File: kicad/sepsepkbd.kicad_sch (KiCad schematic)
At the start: 47 parts, among them J1 MJ-4PP-9, J2 Conn_01x04_Socket, J3 Conn_01x04_Socket, SW1 SW_PUSH, SW10 SW_PUSH, SW11 SW_PUSH, SW12 SW_PUSH, SW13 SW_PUSH, SW14 SW_PUSH, SW15 SW_PUSH, SW16 SW_PUSH, SW17 SW_PUSH, SW18 SW_PUSH, SW19 SW_PUSH, SW2 SW_PUSH, SW20 SW_PUSH, SW21 SW_PUSH, SW3 SW_PUSH, SW4 SW_PUSH, SW5 SW_PUSH, SW6 SW_PUSH, SW7 SW_PUSH, SW8 SW_PUSH, SW9 SW_PUSH, U1 ProMicro

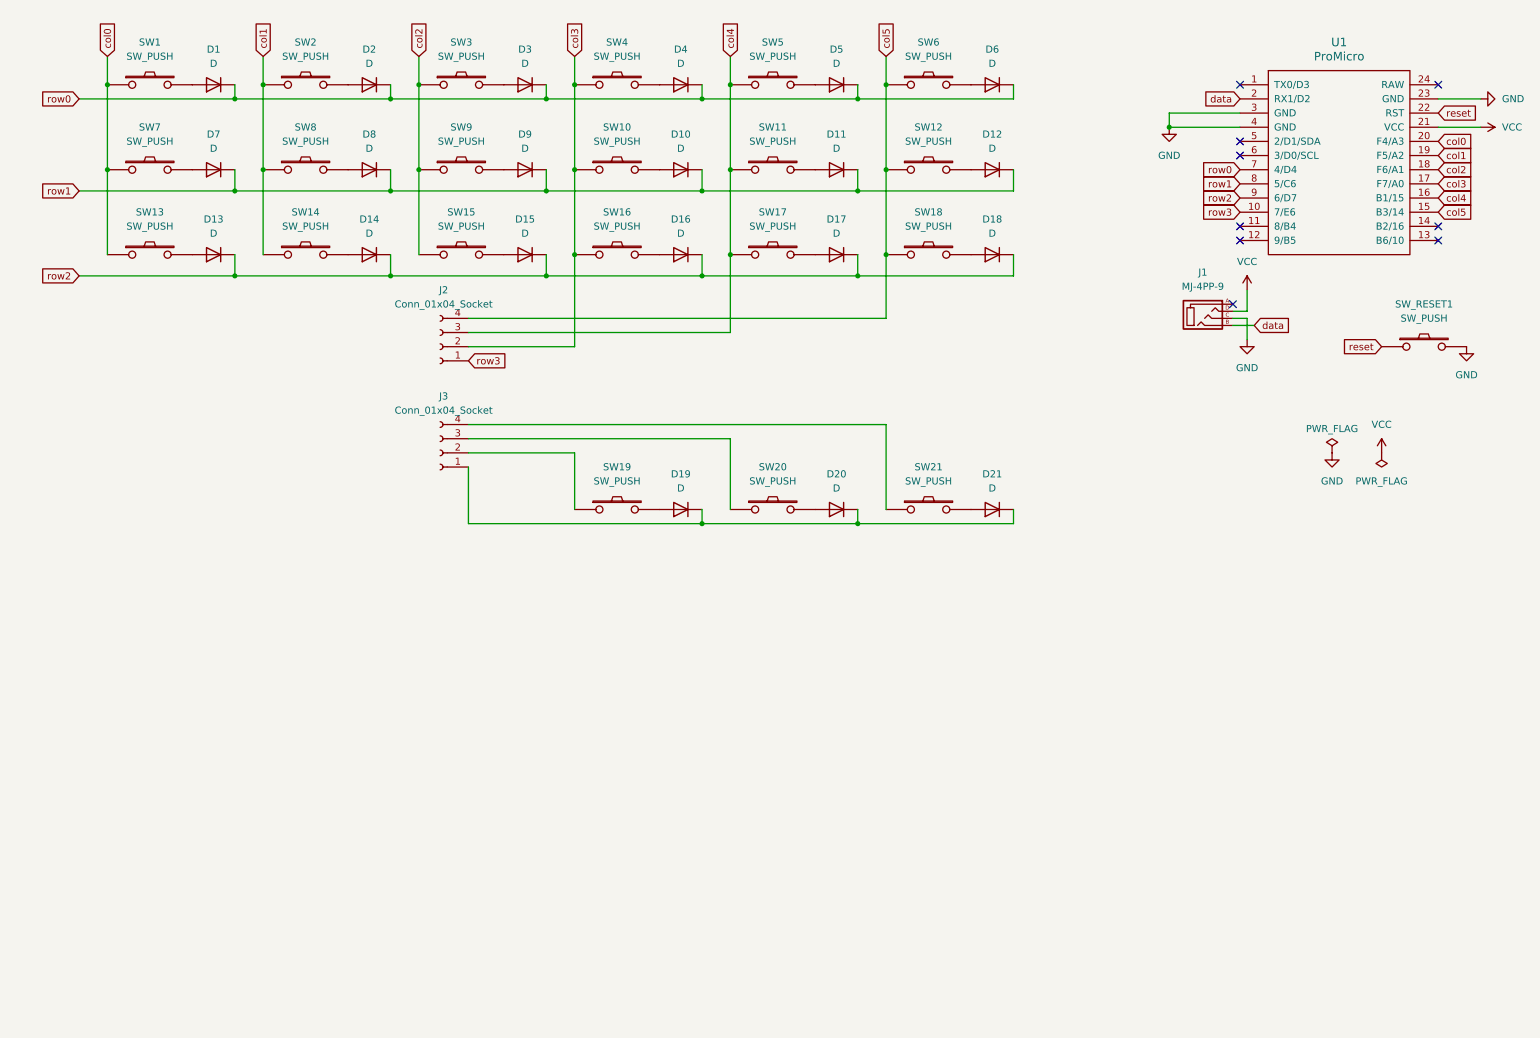
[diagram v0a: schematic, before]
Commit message: 2.1
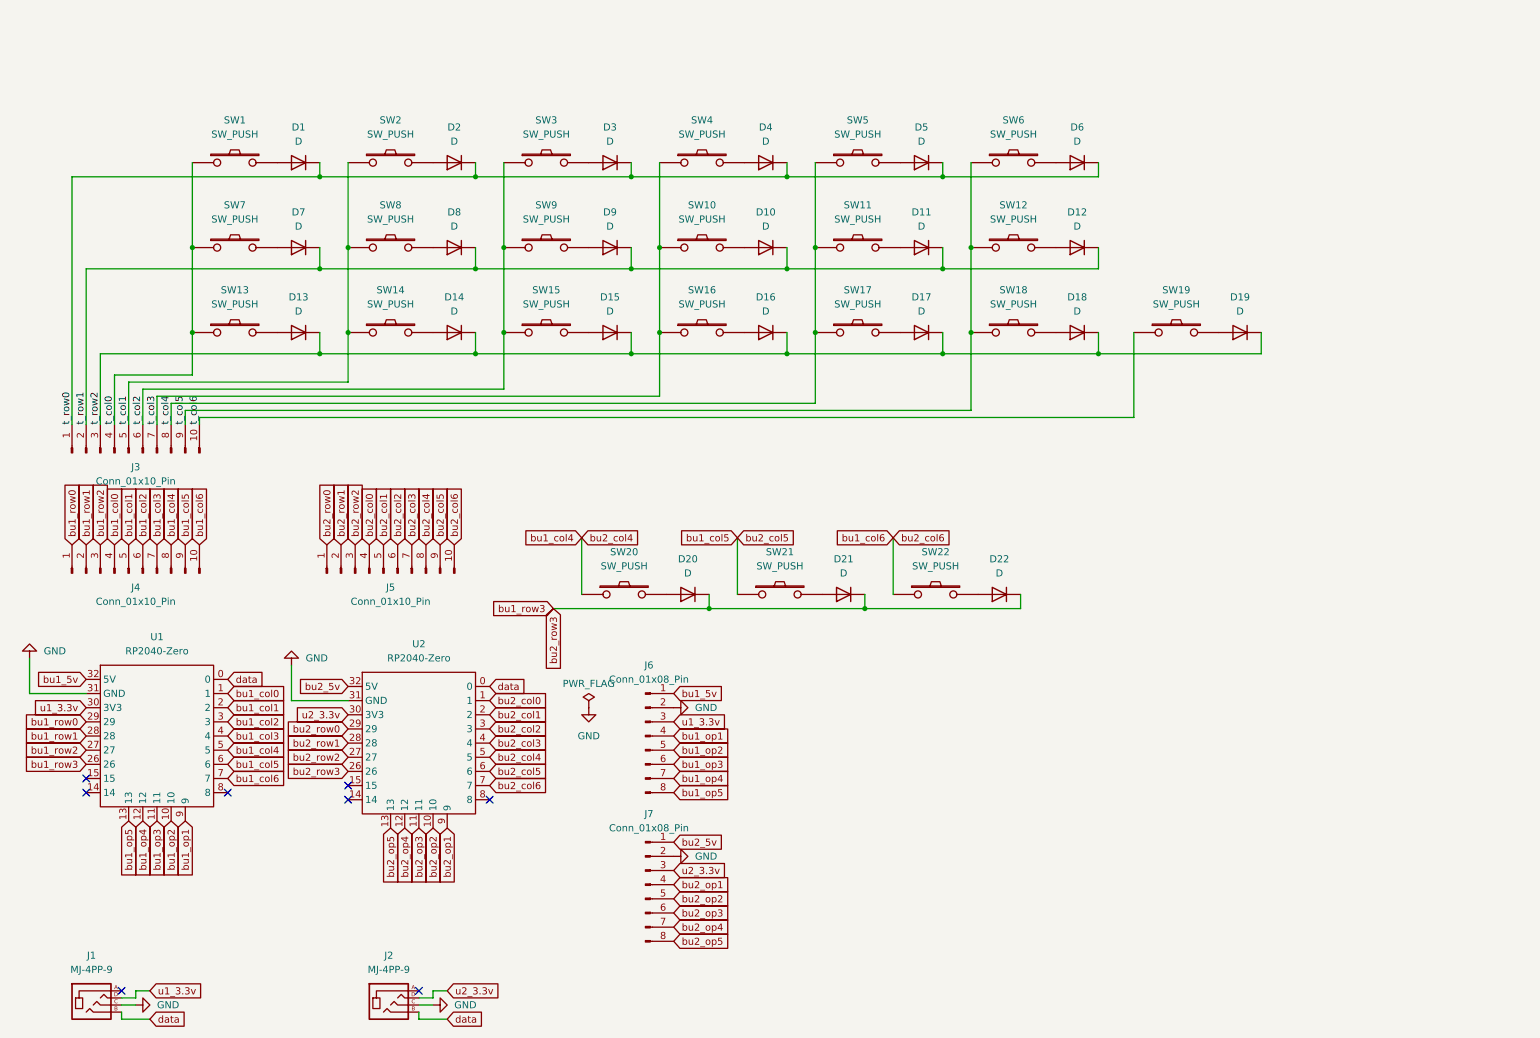
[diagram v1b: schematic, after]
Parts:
- removed J2, J3: Conn_01x04_Socket, Connector_PinHeader_2.54mm:PinHeader_1x04_P2.54mm_Horizontal, symbol Connector:Conn_01x04_Socket
- removed SW_RESET1: SW_PUSH, kbd:ResetSW, symbol kbd:SW_PUSH
- removed U1: ProMicro, kbd:ProMicro_v2, symbol kbd:ProMicro
- added D19: D, kbd:D3_SMD, symbol Device:D
- added J2: MJ-4PP-9, kbd:MJ-4PP-9_1side, symbol kbd:MJ-4PP-9
- added J3, J4, J5: Conn_01x10_Pin, Connector_PinHeader_2.54mm:PinHeader_1x10_P2.54mm_Vertical, symbol Connector:Conn_01x10_Pin
- added J6, J7: Conn_01x08_Pin, Connector_PinHeader_2.54mm:PinHeader_1x08_P2.54mm_Vertical, symbol Connector:Conn_01x08_Pin
- added SW19: SW_PUSH, kbd:ResetSW, symbol kbd:SW_PUSH
- added U1, U2: RP2040-Zero, isw-kbd:RP2040-Zero-THT, symbol isw-mcu:RP2040-Zero
- D20: renamed from D19; footprint kbd:D3_SMD -> kbd:D3_SMD_v2
- D21: renamed from D20; footprint kbd:D3_SMD -> kbd:D3_SMD_v2
- D22: renamed from D21; footprint kbd:D3_SMD -> kbd:D3_SMD_v2
- J1: footprint kbd:MJ-4PP-9 -> kbd:MJ-4PP-9_1side
- SW1, SW10, SW11, SW12, SW13, SW14, SW15, SW16, SW17, SW18, SW2, SW3, SW4, SW5, SW6, SW7, SW8, SW9: footprint keyswitches:SW_PG1350_reversible -> keyswitches:Kailh_socket_PG1350_reversible
- SW20: renamed from SW19; footprint keyswitches:SW_PG1350_reversible -> keyswitches:Kailh_socket_PG1350
- SW21: renamed from SW20; footprint keyswitches:SW_PG1350_reversible -> keyswitches:Kailh_socket_PG1350
- SW22: renamed from SW21; footprint keyswitches:SW_PG1350_reversible -> keyswitches:Kailh_socket_PG1350
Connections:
- net GND: now also J2.C, J6.2 (Pin_2), J7.2 (Pin_2), U1.31 (GND), U2.31 (GND)
- net data: now also J2.B, U1.0, U2.0
- net bu1_col4: now reaches SW20.1
- net bu1_col4: now also J4.8 (Pin_8), J5.8 (Pin_8), U1.5, U2.5
- net bu1_row3: now reaches D20.1 (K), D21.1 (K), D22.1 (K)
- net bu1_row3: now also U1.26, U2.26
- net bu1_col6: now reaches SW22.1
- net bu1_col6: now also J4.10 (Pin_10), J5.10 (Pin_10), U1.7, U2.7
- net bu1_col5: now reaches SW21.1
- net bu1_col5: now also J4.9 (Pin_9), J5.9 (Pin_9), U1.6, U2.6
- net VCC renamed u1_3.3v
- net u1_3.3v: now also J6.3 (Pin_3), U1.30 (3V3)
- net col0 renamed t_col0
- net t_col0: now also J3.4 (Pin_4)
- net col1 renamed t_col1
- net t_col1: now also J3.5 (Pin_5)
- net col2 renamed t_col2
- net t_col2: now also J3.6 (Pin_6)
- net col3 renamed t_col3
- net t_col3: now also J3.7 (Pin_7)
- net col4 renamed t_col4
- net t_col4: now also J3.8 (Pin_8)
- net col5 renamed t_col5
- net t_col5: now also J3.9 (Pin_9)
- net row0 renamed t_row0
- net t_row0: now also J3.1 (Pin_1)
- net row1 renamed t_row1
- net t_row1: now also J3.2 (Pin_2)
- net row2 renamed t_row2
- net t_row2: now also D19.1 (K), J3.3 (Pin_3)
- new net: D19.2 (A), SW19.2
- new net bu1_5v: J6.1 (Pin_1), U1.32 (5V)
- new net bu1_col0: J4.4 (Pin_4), U1.1
- new net bu1_col1: J4.5 (Pin_5), U1.2
- new net bu1_col2: J4.6 (Pin_6), U1.3
- new net bu1_col3: J4.7 (Pin_7), U1.4
- new net bu1_op1: J6.4 (Pin_4), U1.9
- new net bu1_op2: J6.5 (Pin_5), U1.10
- new net bu1_op3: J6.6 (Pin_6), U1.11
- new net bu1_op4: J6.7 (Pin_7), U1.12
- new net bu1_op5: J6.8 (Pin_8), U1.13
- new net bu1_row0: J4.1 (Pin_1), U1.29
- new net bu1_row1: J4.2 (Pin_2), U1.28
- new net bu1_row2: J4.3 (Pin_3), U1.27
- new net bu2_5v: J7.1 (Pin_1), U2.32 (5V)
- new net bu2_col0: J5.4 (Pin_4), U2.1
- new net bu2_col1: J5.5 (Pin_5), U2.2
- new net bu2_col2: J5.6 (Pin_6), U2.3
- new net bu2_col3: J5.7 (Pin_7), U2.4
- new net bu2_op1: J7.4 (Pin_4), U2.9
- new net bu2_op2: J7.5 (Pin_5), U2.10
- new net bu2_op3: J7.6 (Pin_6), U2.11
- new net bu2_op4: J7.7 (Pin_7), U2.12
- new net bu2_op5: J7.8 (Pin_8), U2.13
- new net bu2_row0: J5.1 (Pin_1), U2.29
- new net bu2_row1: J5.2 (Pin_2), U2.28
- new net bu2_row2: J5.3 (Pin_3), U2.27
- new net t_col6: J3.10 (Pin_10), SW19.1
- new net u2_3.3v: J2.D, J7.3 (Pin_3), U2.30 (3V3)
- no-connect marks 9 -> 8
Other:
- moved on the sheet: D1, D10, D11, D12, D13, D14, D15, D16, D17, D18, D2, D20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

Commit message: sep sep -> sprout bird
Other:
- title: now thinking -> Sprout bird
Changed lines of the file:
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@@
 	(paper "A4")
 	(title_block
-		(title "now thinking")
+		(title "Sprout bird")
 		(rev "2.00")
 	)
